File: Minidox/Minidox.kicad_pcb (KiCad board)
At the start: 2 copper layers, 81.8 x 122.2 mm, 53 parts, among them J2 USB_C_Receptacle_USB2.0, SW1 SW_Push, SW3 RotaryEncoder_Switch, U1 ATmega32U4-A, Y1 Crystal_GND24_Small

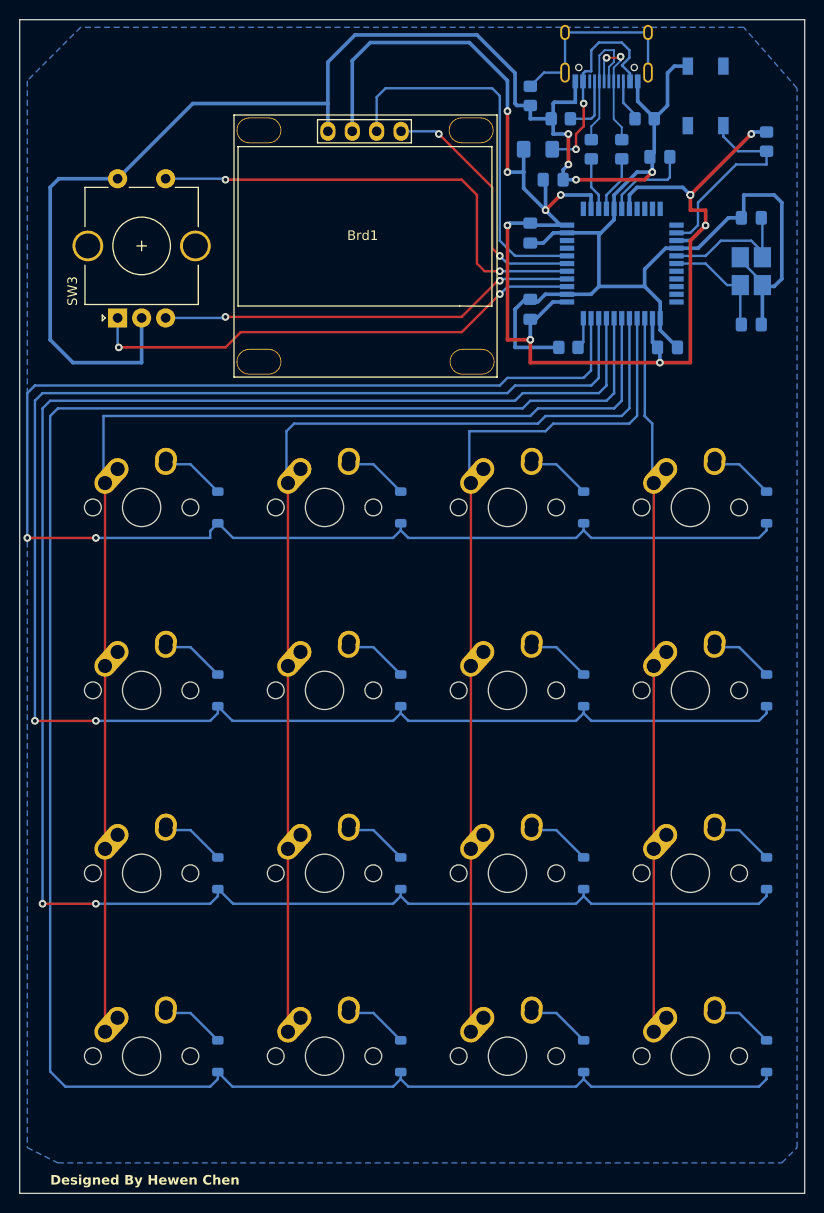
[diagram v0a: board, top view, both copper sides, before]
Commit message: Absonity
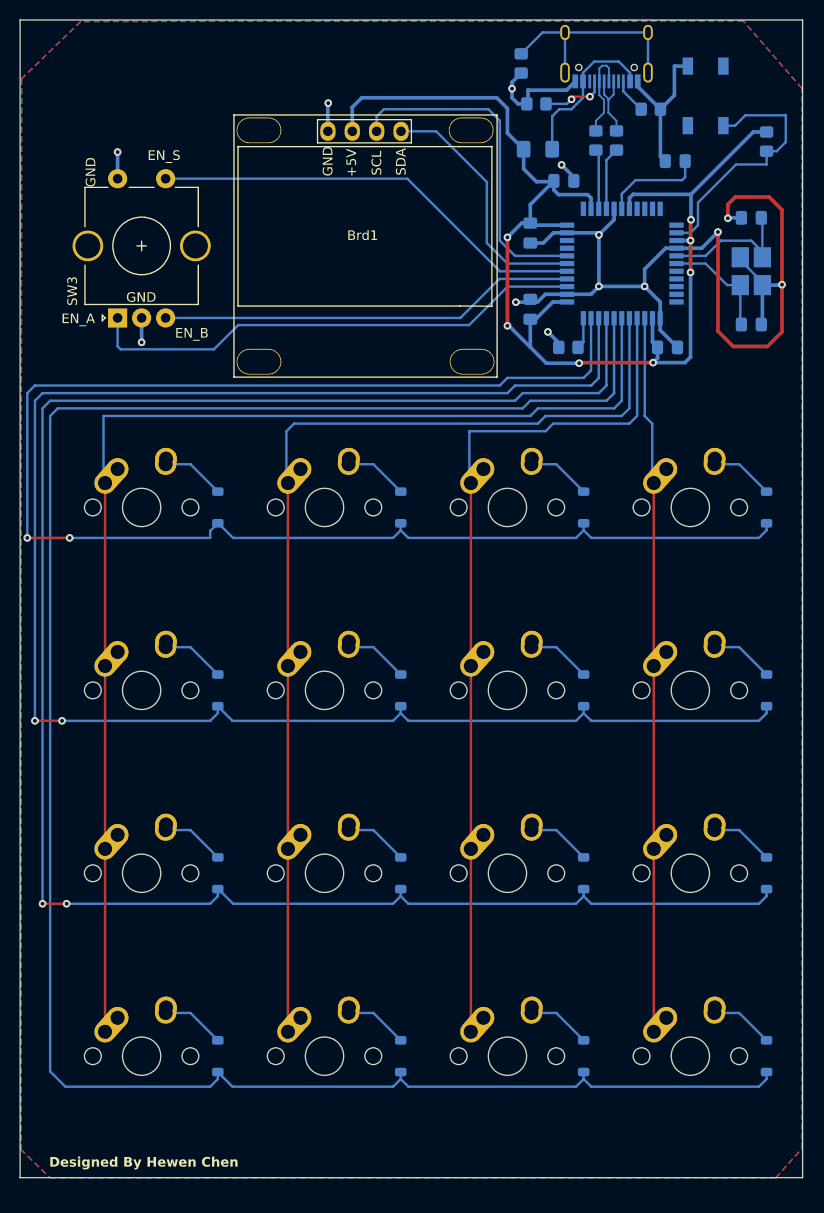
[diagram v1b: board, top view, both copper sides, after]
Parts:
- moved R10 3.51 mm to (115.7, 52.2)
- moved R9 2.97 mm to (117.3, 56.4)
- moved C1 1.66 mm to (131.8, 62.4)
- moved R8 1.18 mm to (129.2, 57.0)
- moved C4 1.12 mm to (120.2, 64.4)
- moved R2 1.06 mm to (125.7, 60.2)
- moved R3 1.03 mm to (123.5, 60.2)
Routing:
- net GND: track 236.9 -> 140.8 mm, vias 4 -> 13
- net +5V: track 151.0 -> 128.2 mm, vias 11 -> 7
- net Net-(U1-~{RESET}): track 21.4 -> 27.2 mm
- net VCC: track 22.4 -> 16.8 mm, vias 2 -> 0
- net D+: track 13.4 -> 7.84 mm, vias 2 -> 0
- net D-: track 14.3 -> 9.67 mm
- net SCL: track 39.8 -> 35.3 mm
- net En_S: track 50.0 -> 45.8 mm, vias 2 -> 0
- net Net-(J2-SHIELD): track 21.2 -> 22.5 mm
- net Net-(U1-UCAP): track 9.35 -> 10.5 mm
- net Net-(J2-CC2): track 4.40 -> 3.67 mm
- net Net-(U1-D-): track 5.53 -> 6.24 mm
- net Net-(U1-D+): track 5.87 -> 6.55 mm
- net En_B: track 44.1 -> 43.5 mm, vias 2 -> 0
- net Net-(J2-CC1): track 6.21 -> 6.68 mm, vias 0 -> 2
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- added copper zone on B.Cu, net GND
- added copper zone on F.Cu, net GND
- removed copper zone on B.Cu, net (none)
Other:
- board size 81.8 x 122.2 mm -> 81.5 x 120.6 mm
- board text added: "+5V"
- board text added: "EN_A"
- board text added: "EN_B"
- board text added: "EN_S"
- board text added: "GND"
- board text added: "SCL"
- board text added: "SDA"
